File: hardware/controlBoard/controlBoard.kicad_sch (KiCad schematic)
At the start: 36 parts, among them J1 Conn_01x10_Pin, J2 USB_C_Receptacle_USB2.0_14P, T1 BC847, T2 BC847, U2 LM1117DT-3.3, U3 CH340G, U4 DS3231M, U5 ESP32-WROOM-32D, Y2 405I35D25M00000

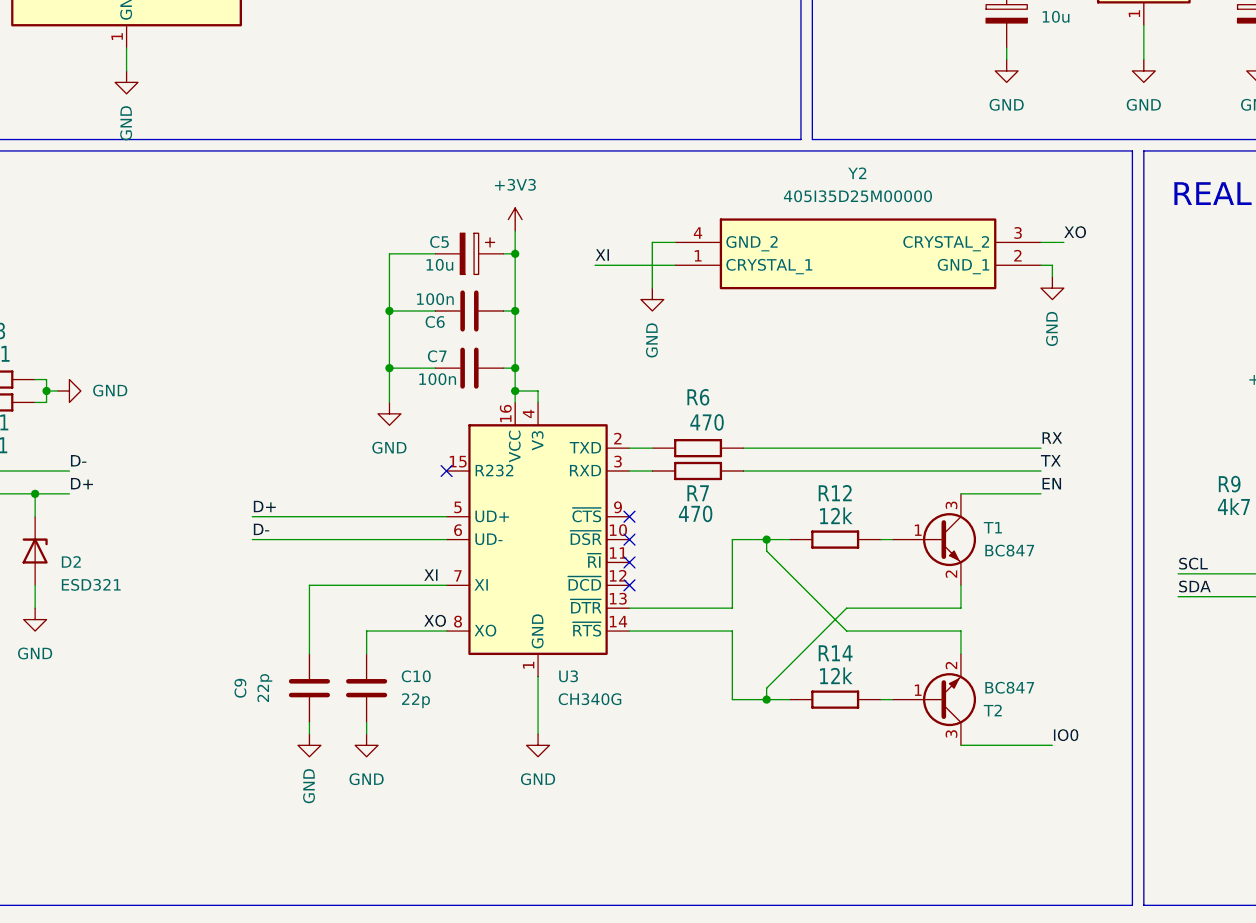
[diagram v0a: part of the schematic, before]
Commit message: Finalize PCB design
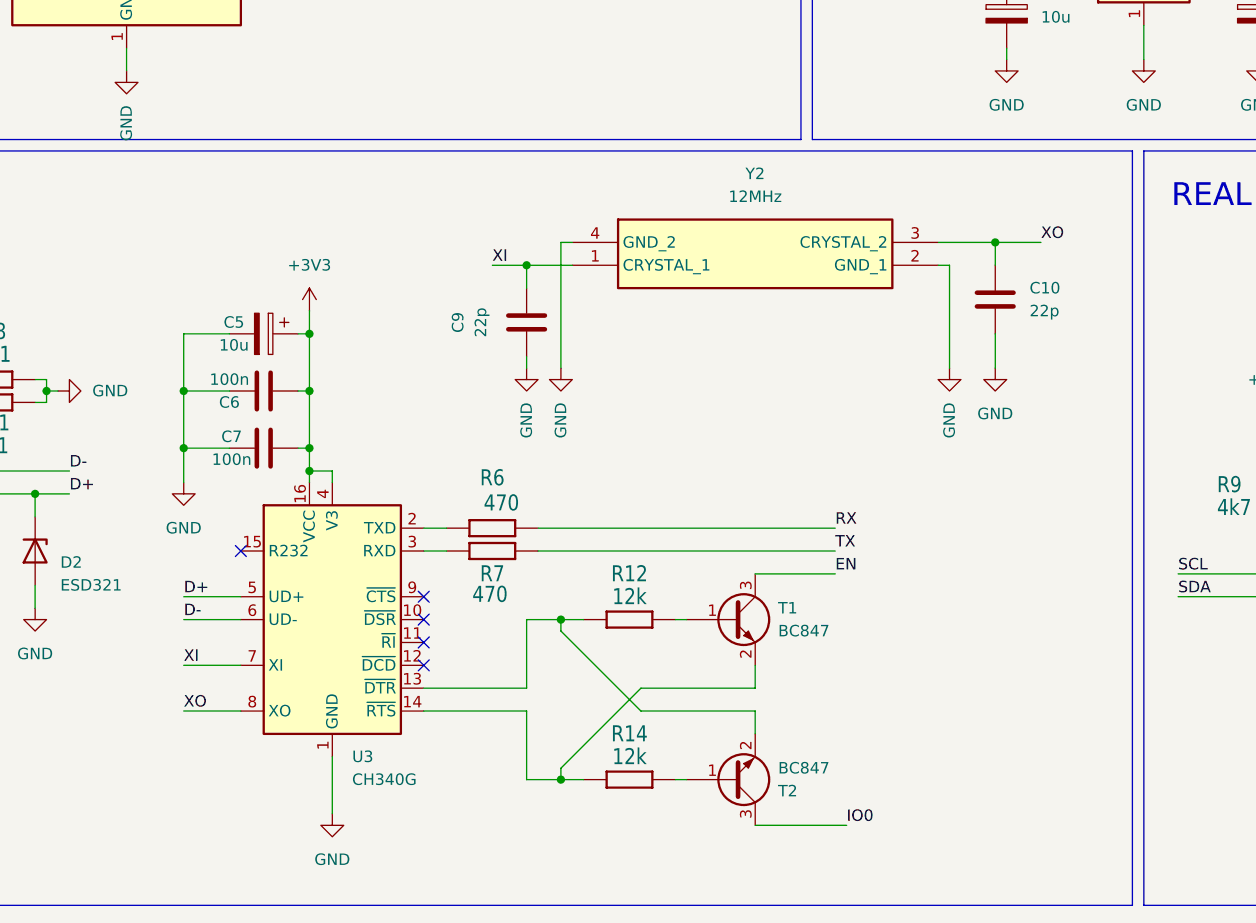
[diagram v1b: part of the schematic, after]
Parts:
- Y2: value 405I35D25M00000 -> 12MHz
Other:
- moved on the sheet: C10, C5, C6, C7, C9, R12, R14, R6, R7, T1, T2, U3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
